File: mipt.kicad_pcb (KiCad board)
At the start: 2 copper layers, 4 parts, among them U1 HLK-7628N, U2 AW9523B, U3 XS2184, U4 BL0910

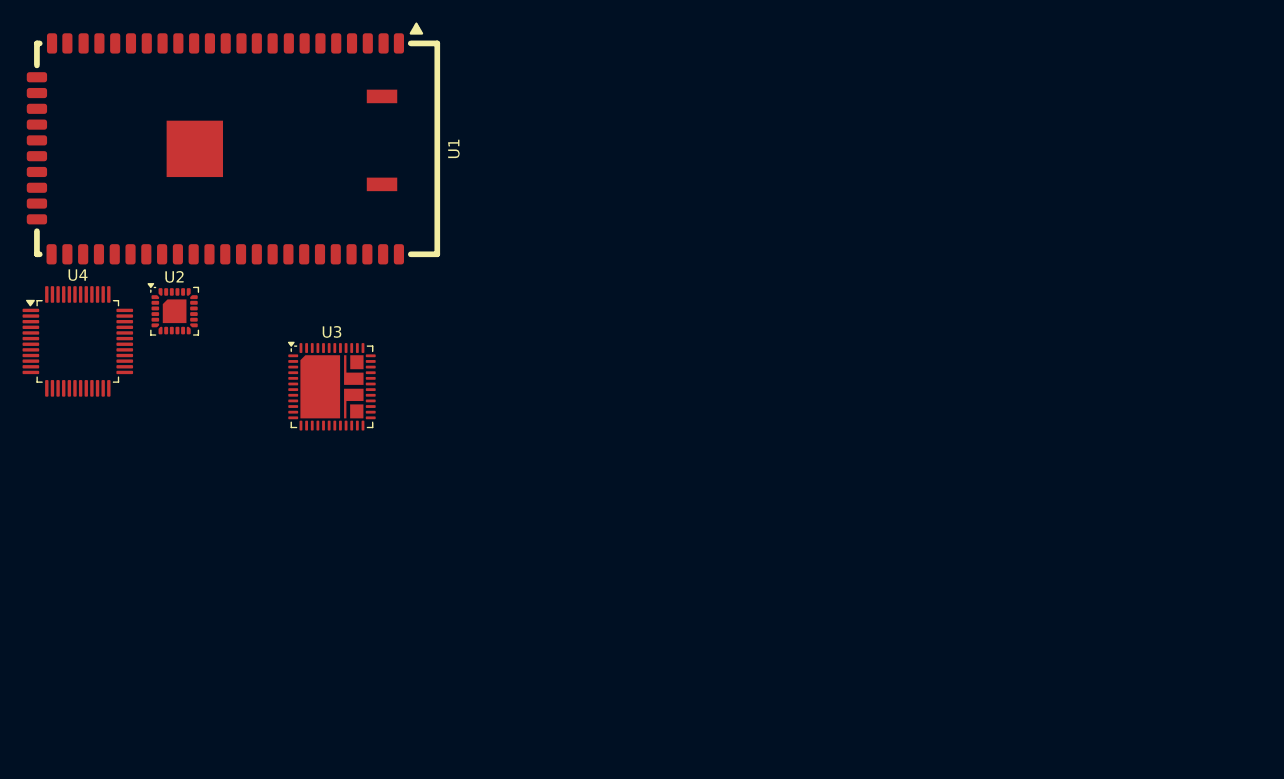
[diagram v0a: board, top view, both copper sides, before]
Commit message: some fixes and add hw 5
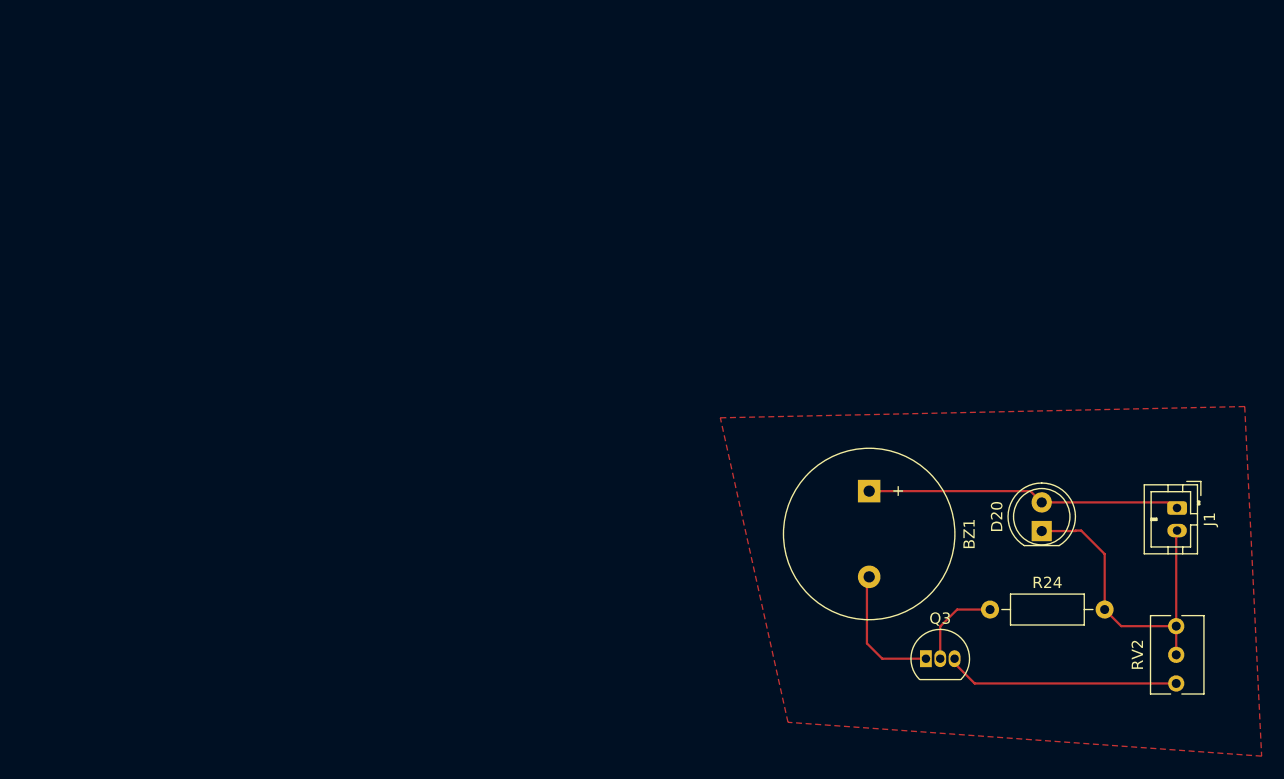
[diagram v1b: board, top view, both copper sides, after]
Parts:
- removed U1: HLK-7628N, mipt:HLK-7628N
- removed U2: AW9523B, mipt:TQFN-24-1EP_4x4mm_P0.5mm_EP2.1x2.1mm
- removed U3: XS2184, mipt:QFN-48-1EP_7x7mm_P0.5mm_EP5.6x5.6mm_1
- removed U4: BL0910, Package_QFP:LQFP-48_7x7mm_P0.5mm
- added BZ1: Buzzer, Buzzer_Beeper:Buzzer_15x7.5RM7.6, F.Cu at (123.2, 87.5)
- added D20: LED, LED_THT:LED_D5.0mm, F.Cu at (138.5, 91.0)
- added J1: Conn_01x02_Pin, Connector_JST:JST_PH_B2B-PH-K_1x02_P2.00mm_Vertical, F.Cu at (150.5, 89.0)
- added Q3: BC337-40, Package_TO_SOT_THT:TO-92_Inline, F.Cu at (128.2, 102.4)
- added R24: R, Resistor_THT:R_Axial_DIN0207_L6.3mm_D2.5mm_P10.16mm_Horizontal, F.Cu at (133.9, 98.0)
- added RV2: R_Potentiometer, Potentiometer_THT:Potentiometer_Bourns_3266Y_Vertical, F.Cu at (150.4, 99.5)
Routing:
- net Net-(D20-K): track 0.00 -> 29.4 mm
- net Net-(BT1-+): track 0.00 -> 27.9 mm
- net Net-(BT1--): track 0.00 -> 20.8 mm
- net Net-(BZ1--): track 0.00 -> 11.8 mm
- net Net-(Q3-B): track 0.00 -> 7.90 mm
- added copper zone on F.Cu, net GND
